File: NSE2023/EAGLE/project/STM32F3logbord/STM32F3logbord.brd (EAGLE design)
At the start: 50 x 50 mm, 49 parts, among them CN1 DM3AT, SW1 SRIDE_SWITCH

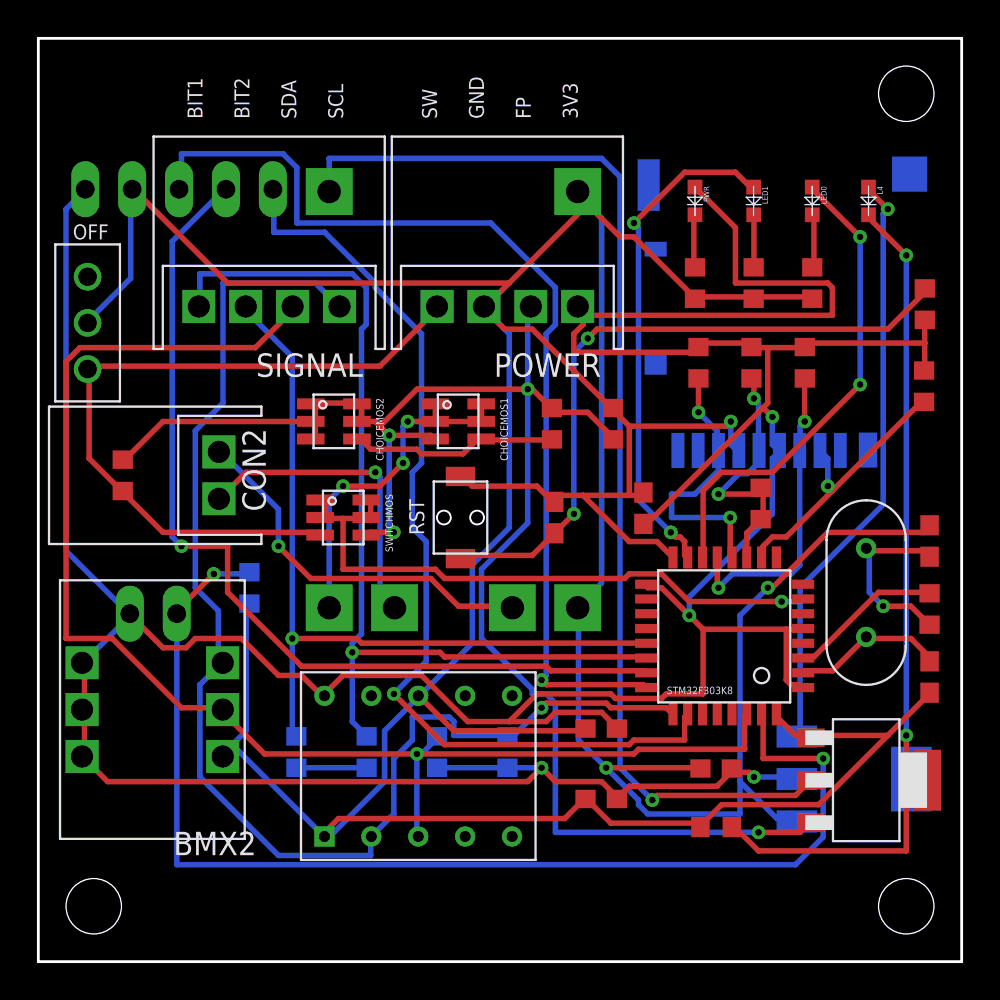
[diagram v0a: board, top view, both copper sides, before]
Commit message: add
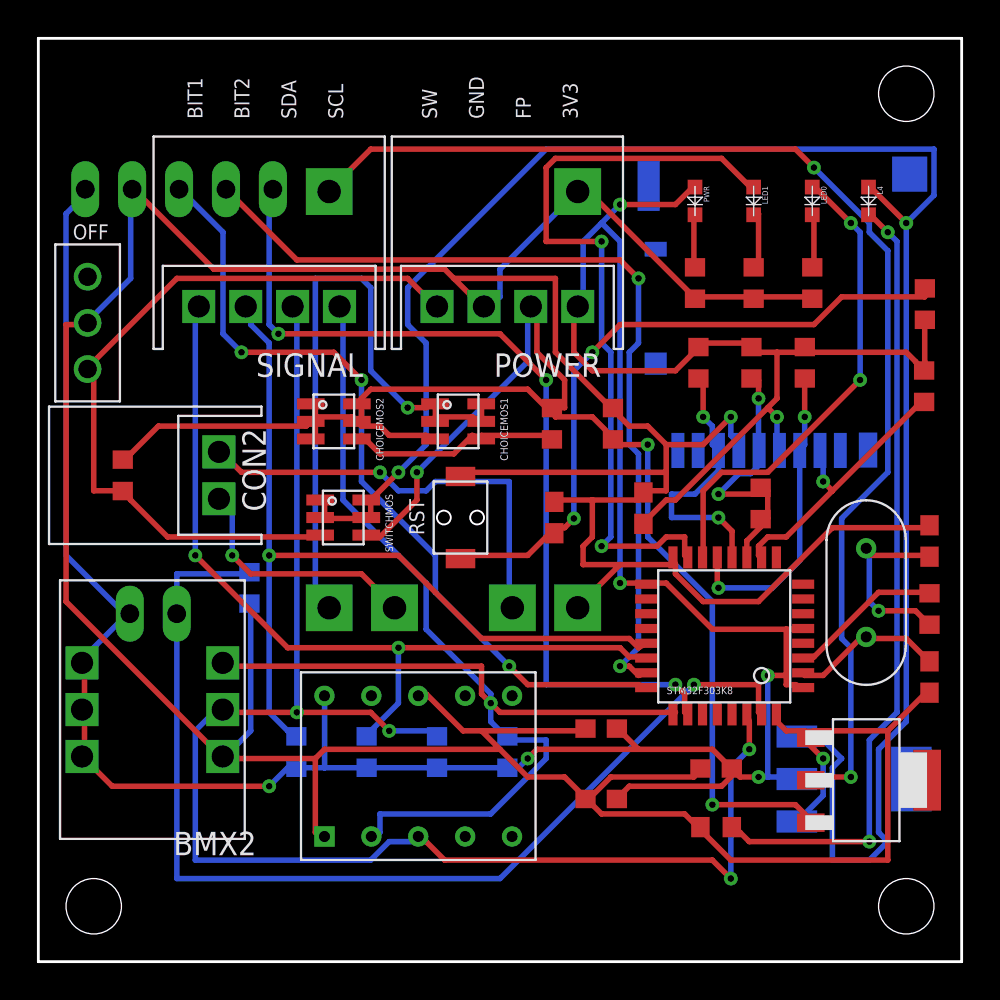
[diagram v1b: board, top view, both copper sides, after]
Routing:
- net +3V3: track 222.0 -> 181.3 mm, vias 4 -> 7
- net N$11: track 65.8 -> 103.8 mm
- net GND: track 271.7 -> 248.1 mm, vias 3 -> 2
- net MAINBATTE: track 18.9 -> 34.6 mm, vias 3 -> 1
- net LED1: track 27.4 -> 41.9 mm
- net SWCLK: track 54.4 -> 44.0 mm, vias 1 -> 3
- net SDA: track 76.2 -> 83.2 mm, vias 1 -> 4
- net BIT1: track 52.1 -> 45.7 mm, vias 1 -> 2
- net BOOT0: track 64.1 -> 58.0 mm, vias 2 -> 1
- net N$5: track 61.5 -> 65.8 mm, vias 1 -> 2
- net N$12: track 16.8 -> 13.4 mm
- net BIT2: track 43.8 -> 47.0 mm
- net N$13: track 20.5 -> 23.7 mm
- net SWO: track 52.0 -> 49.0 mm, vias 1 -> 3
- net SWDIO: track 50.2 -> 47.8 mm, vias 1 -> 2
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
